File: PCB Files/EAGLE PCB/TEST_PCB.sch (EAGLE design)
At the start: 19 parts, among them IC1 4066D, IC2 OP-AMP

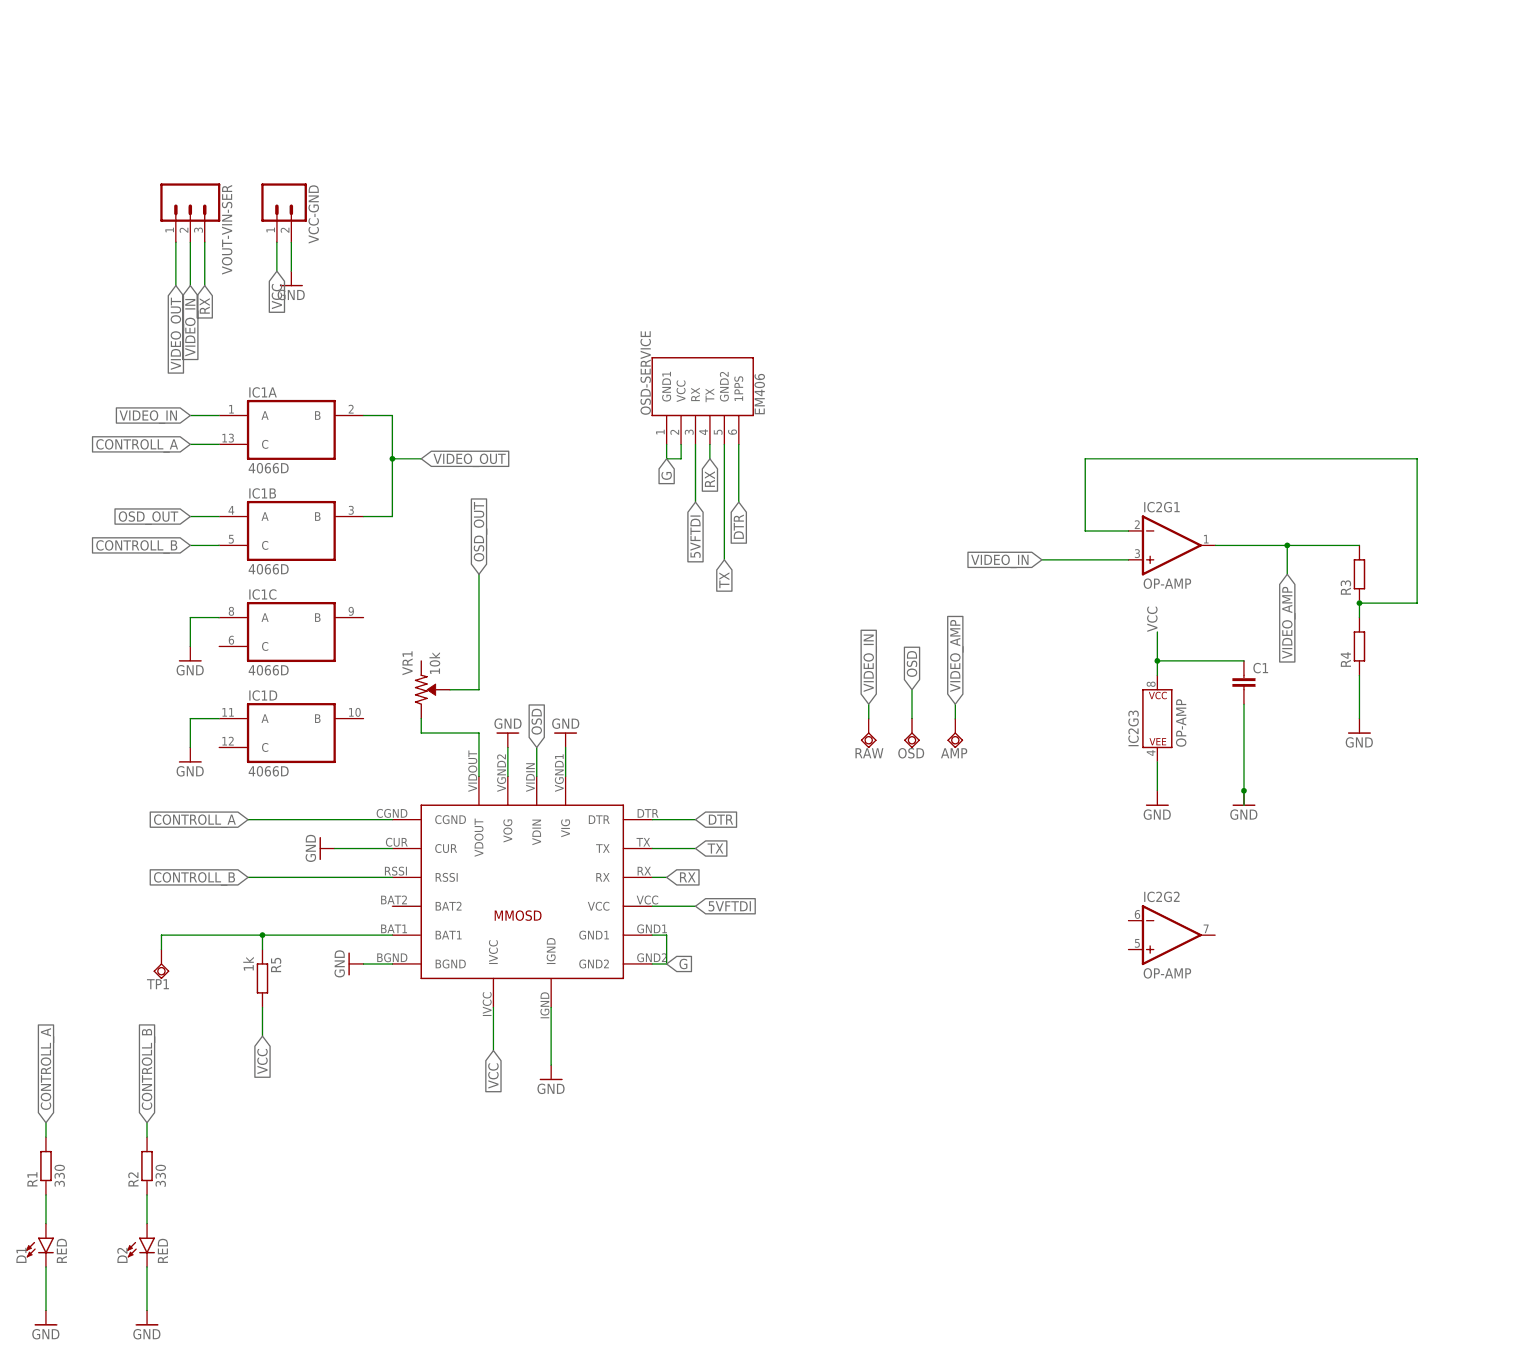
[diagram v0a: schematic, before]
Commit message: Experimental PCBs
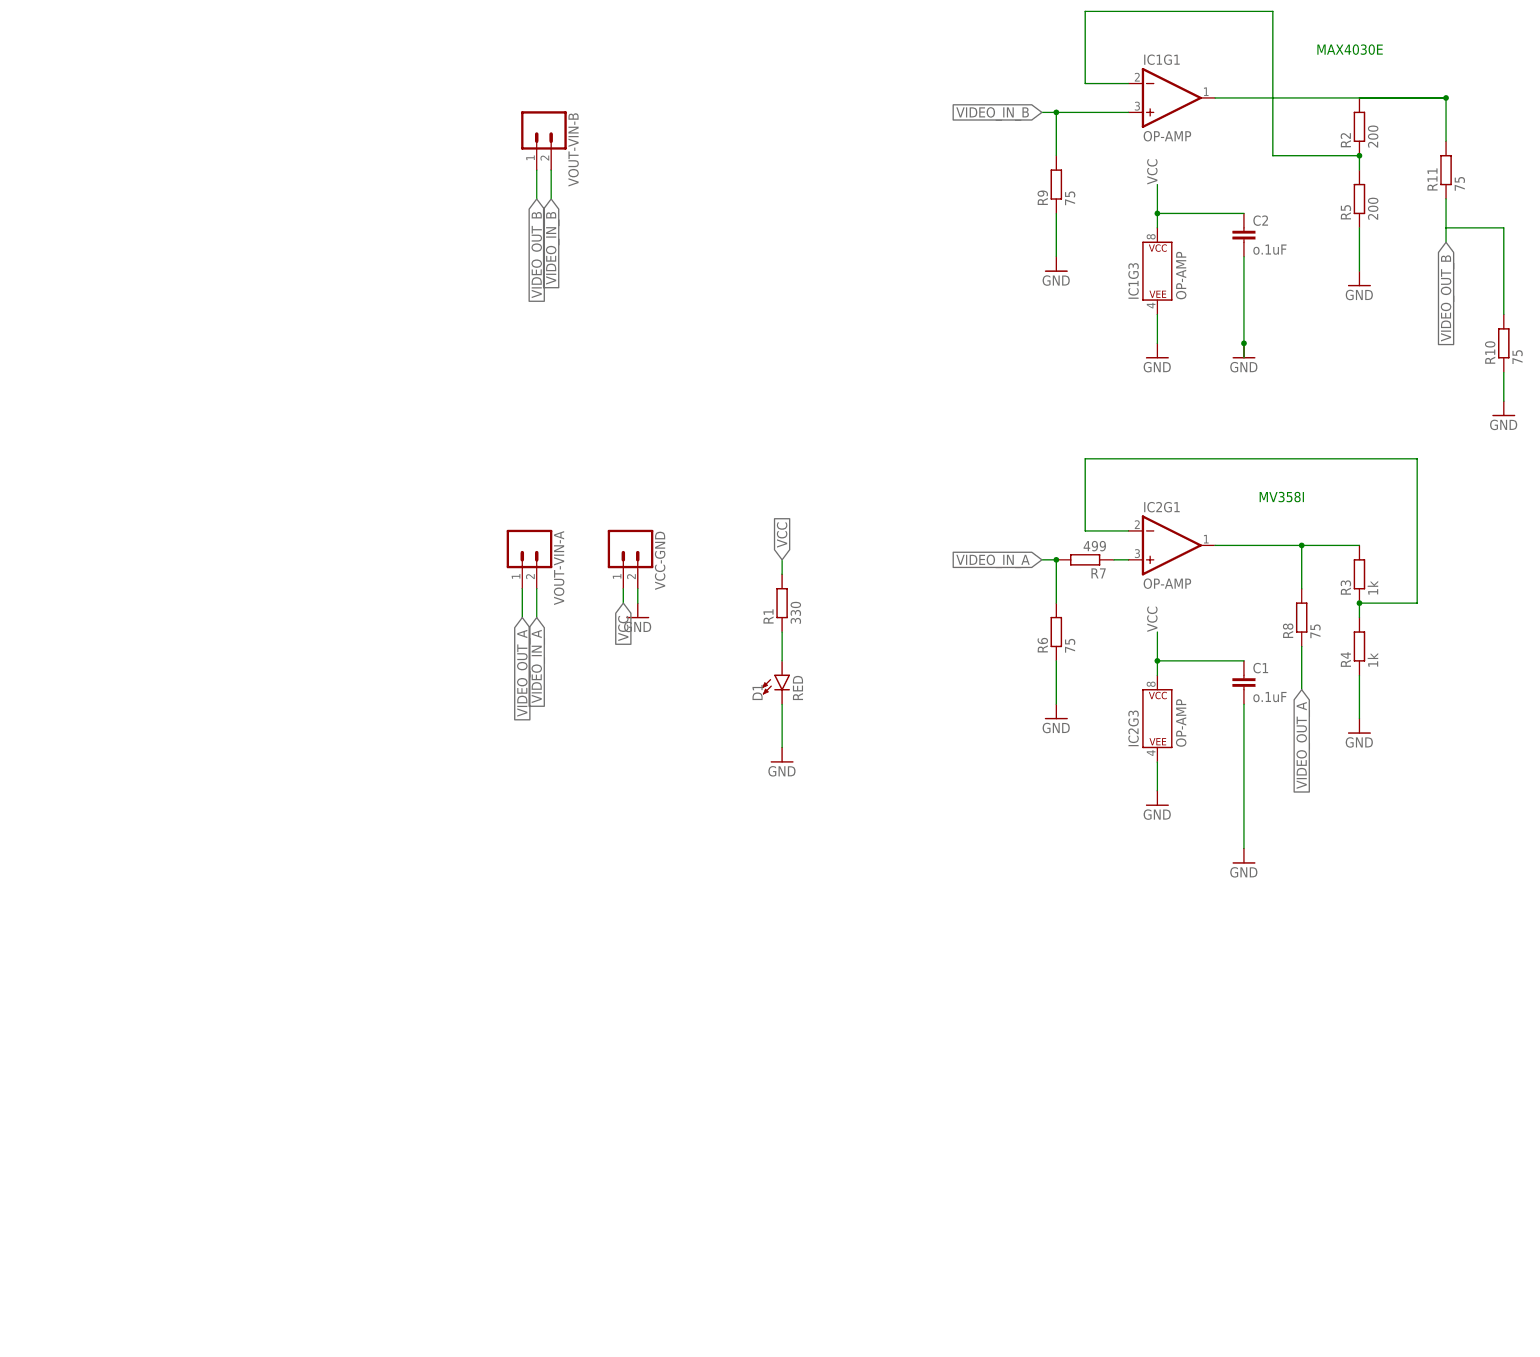
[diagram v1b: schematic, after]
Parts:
- removed AMP, OSD, RAW, TP1: TPSQTP13SQ, testpad:TPSQTP13SQ
- removed D2: RED, SparkFun-LED:LED-RED1206
- removed MINIMOSD: MICROMINIMOSDPWR, FPVTools:MICROMINIMOSDPWR
- removed OSD-SERVICE: EM406, SparkFun-Connectors:EM406
- removed VOUT-VIN-SER: (no value), SparkFun-Connectors:CONN_03
- removed VR1: 10k, SparkFun-Resistors:TRIMPOT-SMD-3MM-CLOSED-1/8W-20%
- added C2: o.1uF, rcl:C-EUC0603K
- added R10, R11, R6, R8, R9: 75, resistor:R-EU_R0603
- added R7: 499, resistor:R-EU_R0603
- added VOUT-VIN-A, VOUT-VIN-B: (no value), SparkFun-Connectors:CONN_02
- C1: value (none) -> o.1uF
- IC1: value 4066D -> OP-AMP; device 40xx:4066D -> SparkFun-IC-Amplifiers:OPAMP-DUALU
- R2: value 330 -> 200
- R3, R4: value (none) -> 1k
- R5: value 1k -> 200
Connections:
- removed net 5VFTDI: MINIMOSD.VCC, OSD-SERVICE.RX
- removed net CONTROLL_A: IC1A.C, MINIMOSD.CGND, R1.2
- removed net CONTROLL_B: IC1B.C, MINIMOSD.RSSI, R2.2
- removed net DTR: MINIMOSD.DTR, OSD-SERVICE.1PPS
- removed net G: MINIMOSD.GND1, MINIMOSD.GND2, OSD-SERVICE.GND1, OSD-SERVICE.VCC
- removed net N$3: MINIMOSD.BAT1, R5.1, TP1.TP
- removed net N$6: MINIMOSD.VDOUT, VR1.CW
- removed net OSD: MINIMOSD.VDIN, OSD.TP
- removed net OSD_OUT: IC1B.A, VR1.WIPER
- removed net RX: MINIMOSD.RX, OSD-SERVICE.TX, VOUT-VIN-SER.3
- removed net TX: MINIMOSD.TX, OSD-SERVICE.GND2
- removed net VIDEO_AMP: AMP.TP, IC2G1.OUT, R3.2
- removed net VIDEO_IN: IC1A.A, IC2G1.+IN, RAW.TP, VOUT-VIN-SER.2
- removed net VIDEO_OUT: IC1A.B, IC1B.B, VOUT-VIN-SER.1
- new net 1: IC1G1.OUT, R11.2, R2.2
- new net 75: IC2G1.OUT, R3.2, R8.2
- new net N$5: IC2G1.+IN, R7.1
- new net VIDEO_IN_A: R6.2, R7.2, VOUT-VIN-A.2
- new net VIDEO_IN_B: IC1G1.+IN, R9.2, VOUT-VIN-B.2
- new net VIDEO_OUT_A: R8.1, VOUT-VIN-A.1
- new net VIDEO_OUT_B: R10.2, R11.1, VOUT-VIN-B.1
- net GND: now also C2.2, IC1G3.P$V-, R10.1, R5.1, R6.1, R9.1; no longer D2.C, IC1C.A, IC1D.A, MINIMOSD.BGND, MINIMOSD.CUR, MINIMOSD.IGND, MINIMOSD.VIG, MINIMOSD.VOG
- net N$1: now also IC1G1.-IN, R5.2; no longer D2.A
- net VCC: now also C2.1, IC1G3.P$V+, R1.2; no longer MINIMOSD.IVCC, R5.2
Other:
- note added: "MAX4030E"
- note added: "MV358I"
- moved on the sheet: D1, R1, R2, R5, VCC-GND
